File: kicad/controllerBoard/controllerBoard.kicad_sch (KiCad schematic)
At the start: 2 parts, among them J1 Conn_02x20_Top_Bottom, J2 Conn_02x20_Top_Bottom

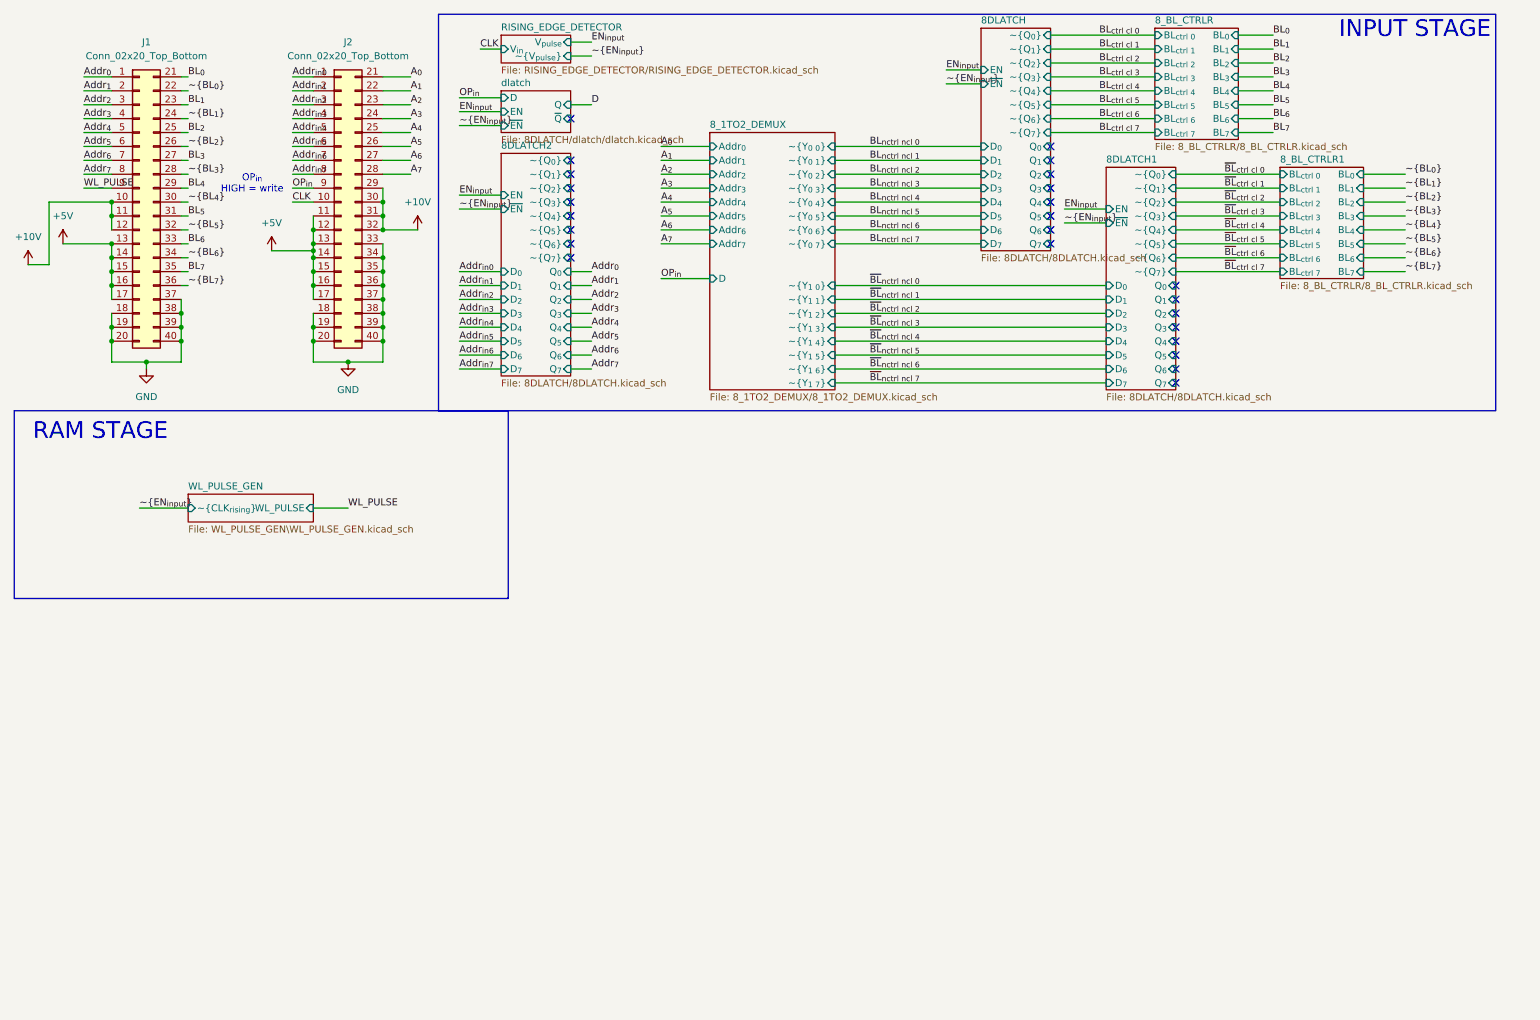
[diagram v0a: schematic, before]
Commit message: finish main schematic
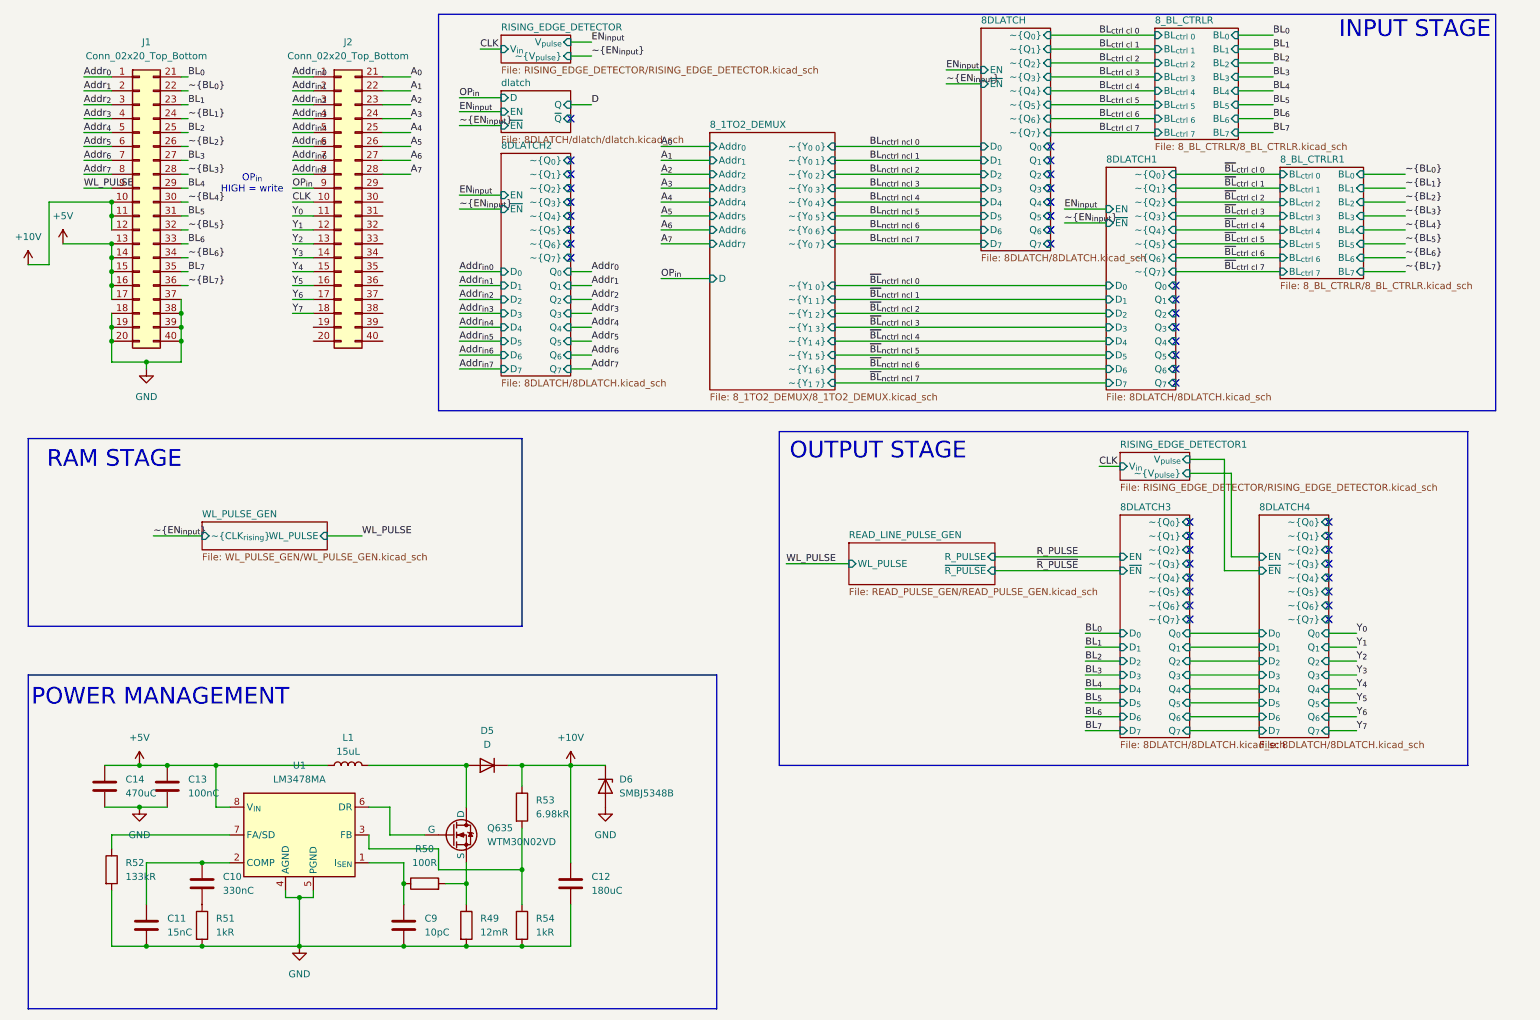
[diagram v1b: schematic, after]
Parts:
- added C10: 330nC, symbol Device:C
- added C11: 15nC, symbol Device:C
- added C12: 180uC, symbol Device:C
- added C13: 100nC, symbol Device:C
- added C14: 470uC, symbol Device:C
- added C9: 10pC, symbol Device:C
- added D5: D, symbol Device:D
- added D6: SMBJ5348B, symbol Device:D_Zener
- added L1: 15uL, symbol Device:L
- added Q635: WTM30N02VD, symbol Simulation_SPICE:NMOS
- added R49: 12mR, symbol Device:R
- added R50: 100R, symbol Device:R
- added R51, R54: 1kR, symbol Device:R
- added R52: 133kR, symbol Device:R
- added R53: 6.98kR, symbol Device:R
- added U1: LM3478MA, Package_SO:SOIC-8_3.9x4.9mm_P1.27mm, symbol Regulator_Controller:LM3478MA
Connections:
- net +10V: now also C12.1, D5.1 (K), D6.1 (K), R53.1; no longer J2.29 (Pin_29), J2.30 (Pin_30), J2.31 (Pin_31), J2.32 (Pin_32)
- net +5V: now also C13.1, C14.1, L1.1, U1.8 (V_{IN}); no longer J2.11 (Pin_11), J2.12 (Pin_12), J2.13 (Pin_13), J2.14 (Pin_14), J2.15 (Pin_15), J2.16 (Pin_16), J2.17 (Pin_17)
- net GND: now also C11.2, C12.2, C13.2, C14.2, C9.2, D6.2 (A), R49.2, R51.2, R52.2, R54.2, U1.4 (AGND), U1.5 (PGND); no longer J2.18 (Pin_18), J2.19 (Pin_19), J2.20 (Pin_20), J2.33 (Pin_33), J2.34 (Pin_34), J2.35 (Pin_35), J2.36 (Pin_36), J2.37 (Pin_37), J2.38 (Pin_38), J2.39 (Pin_39), J2.40 (Pin_40)
- new net: R53.2, R54.1, U1.3 (FB)
- new net: C10.1, C11.1, U1.2 (COMP)
- new net: Q635.3 (S), R49.1, R50.2
- new net: D5.2 (A), L1.2, Q635.1 (D)
- new net: Q635.2 (G), U1.6 (DR)
- new net: C9.1, R50.1, U1.1 (I_{SEN})
- new net: R52.1, U1.7 (FA/SD)
- new net: C10.2, R51.1
- new net Y_{0}: J2.11 (Pin_11)
- new net Y_{1}: J2.12 (Pin_12)
- new net Y_{2}: J2.13 (Pin_13)
- new net Y_{3}: J2.14 (Pin_14)
- new net Y_{4}: J2.15 (Pin_15)
- new net Y_{5}: J2.16 (Pin_16)
- new net Y_{6}: J2.17 (Pin_17)
- new net Y_{7}: J2.18 (Pin_18)
- no-connect marks 25 -> 41
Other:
- added sheet 8DLATCH3 (8DLATCH/8DLATCH.kicad_sch)
- added sheet 8DLATCH4 (8DLATCH/8DLATCH.kicad_sch)
- added sheet READ_LINE_PULSE_GEN (READ_PULSE_GEN/READ_PULSE_GEN.kicad_sch)
- added sheet RISING_EDGE_DETECTOR1 (RISING_EDGE_DETECTOR/RISING_EDGE_DETECTOR.kicad_sch)
- sheet WL_PULSE_GEN: file WL_PULSE_GEN\WL_PULSE_GEN.kicad_sch -> WL_PULSE_GEN/WL_PULSE_GEN.kicad_sch
- note added: "OUTPUT STAGE"
- note added: "POWER MANAGEMENT"
